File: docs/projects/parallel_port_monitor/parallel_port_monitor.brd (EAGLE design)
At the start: 51.1 x 61 mm, 22 parts

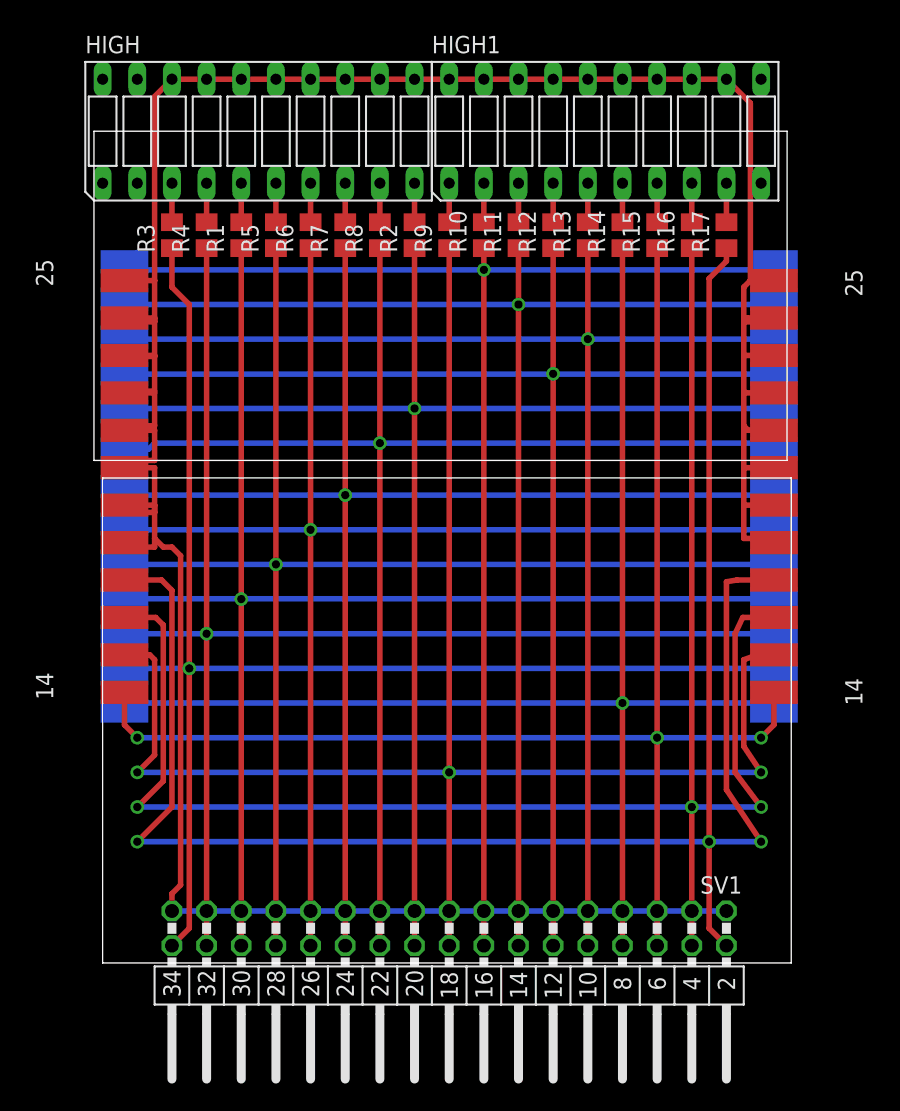
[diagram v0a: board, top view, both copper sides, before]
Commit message: fix airwires
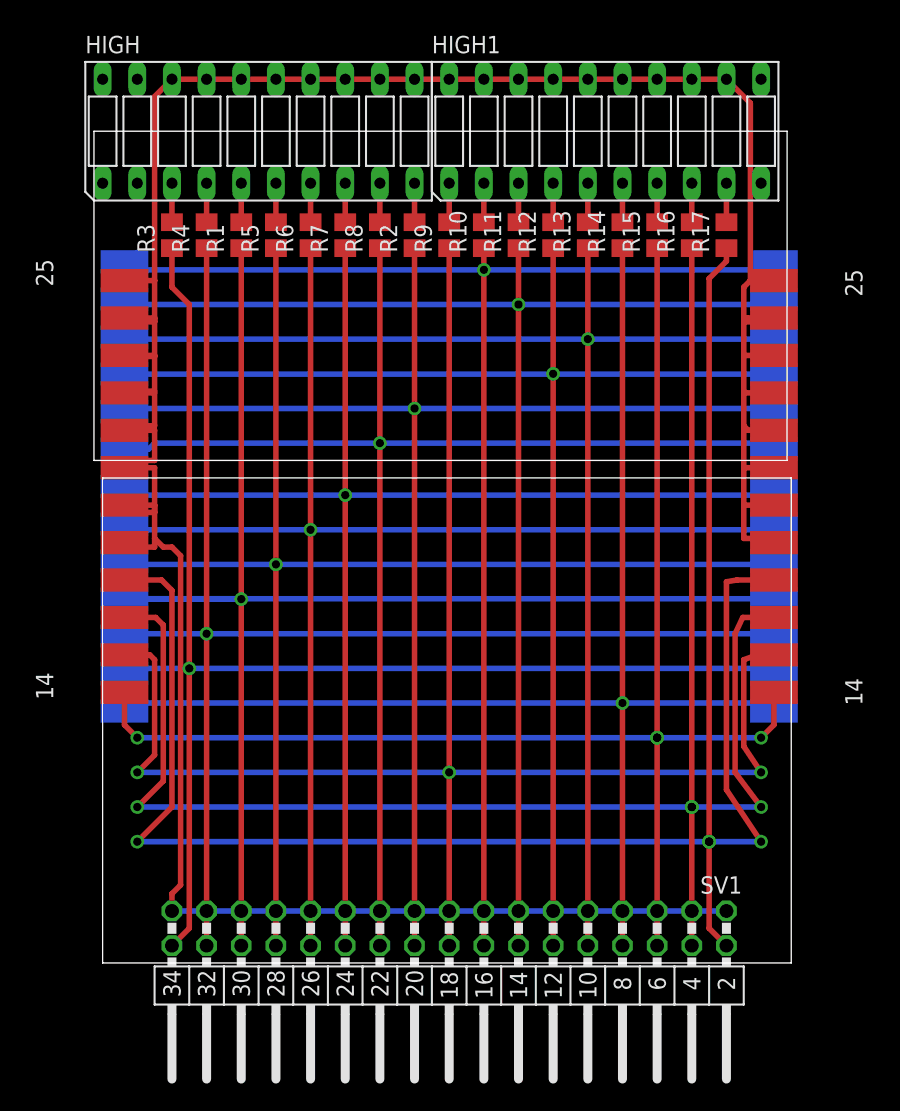
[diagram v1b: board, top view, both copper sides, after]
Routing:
- net C1: track 58.6 -> 104.3 mm, vias 0 -> 4
- net S3: track 73.2 -> 118.9 mm, vias 0 -> 3
- net N$26: track 45.7 -> 0.00 mm, vias 3 -> 0
- net N$24: track 45.7 -> 0.00 mm, vias 3 -> 0
- net N$23: track 45.7 -> 0.00 mm, vias 3 -> 0
- net N$21: track 45.7 -> 0.00 mm, vias 3 -> 0
- net C3: track 98.7 -> 144.5 mm, vias 0 -> 4
- net C2: track 85.3 -> 131.0 mm, vias 0 -> 4
- net DATA2: track 98.7 -> 107.3 mm, vias 0 -> 1
- net S6: vias 0 -> 1
